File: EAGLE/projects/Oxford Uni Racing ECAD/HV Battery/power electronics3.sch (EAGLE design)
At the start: 57 parts, among them IC1 4043N, IC2 4001N, IC3 LM555CN, IC4 4071N, IC5 4081N, IC6 4011N, IC7 4011N, K1 T9AS1D12-48=T9A, K2 T9AS5D12-12=T9A, K4 T9AS1D12-48=T9A, K5 T9AS1D12-48=T9A, Q1 BS170, Q2 BS170, Q3 BS170

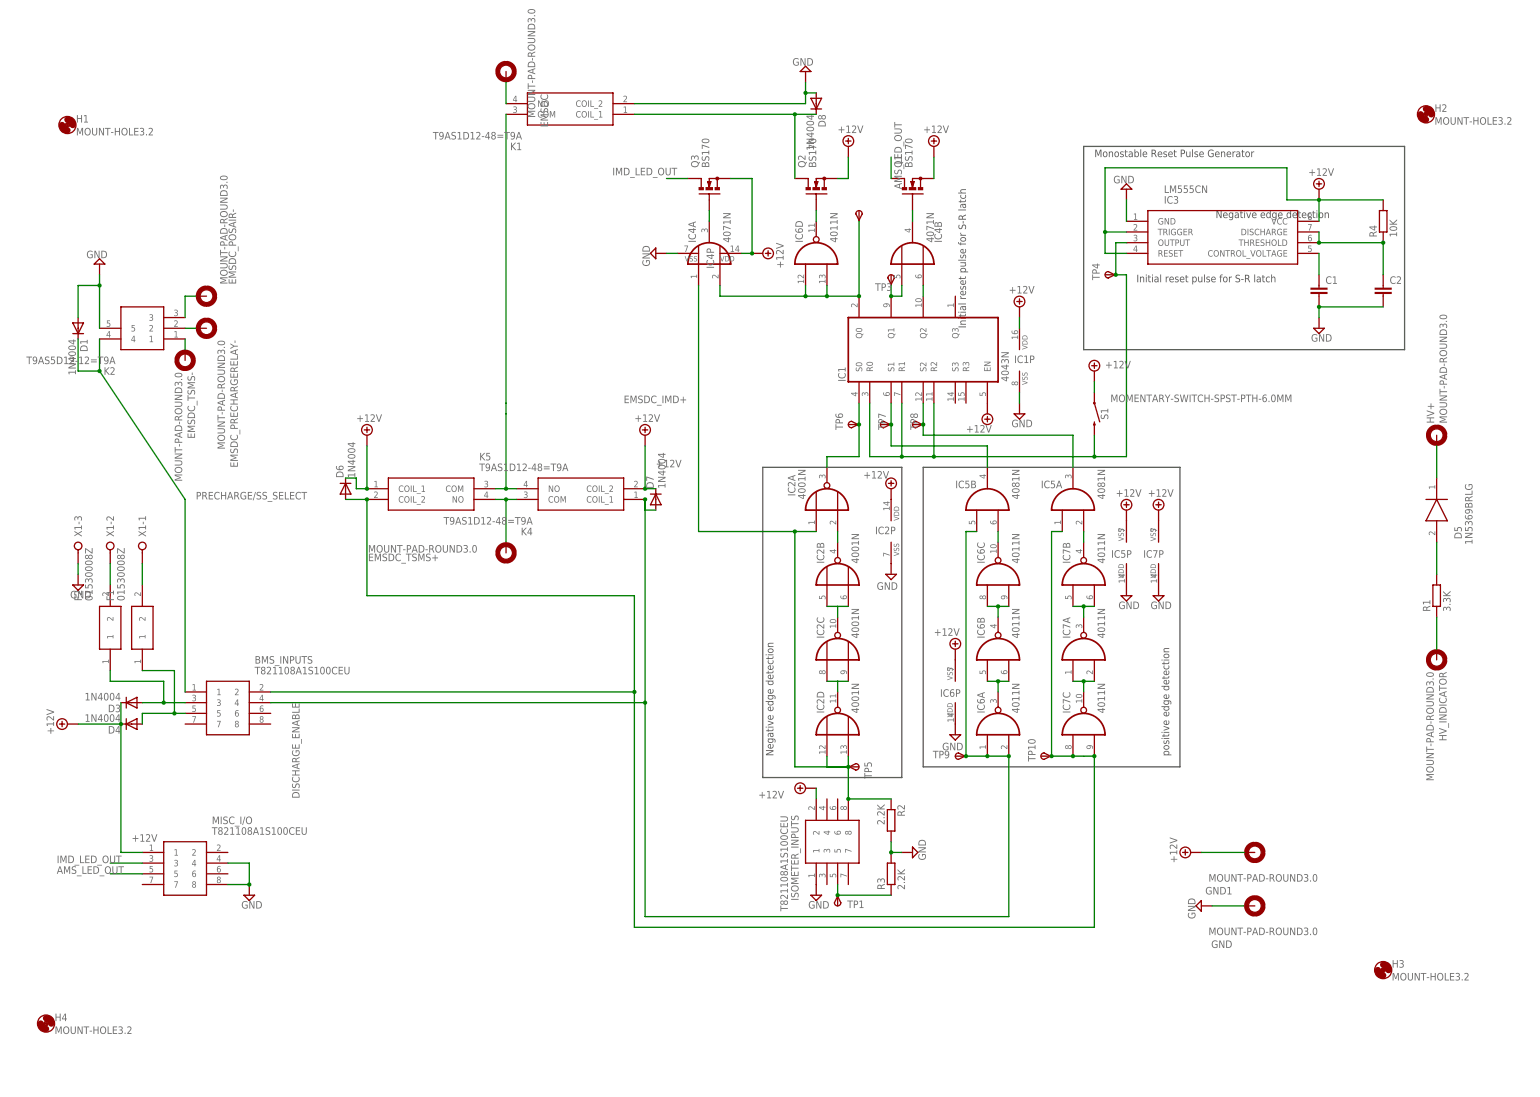
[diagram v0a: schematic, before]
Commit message: Modifications suggested by Dan after first review
Signed-off-by: Jack Bruford <jack.bruford41@gmail.com>
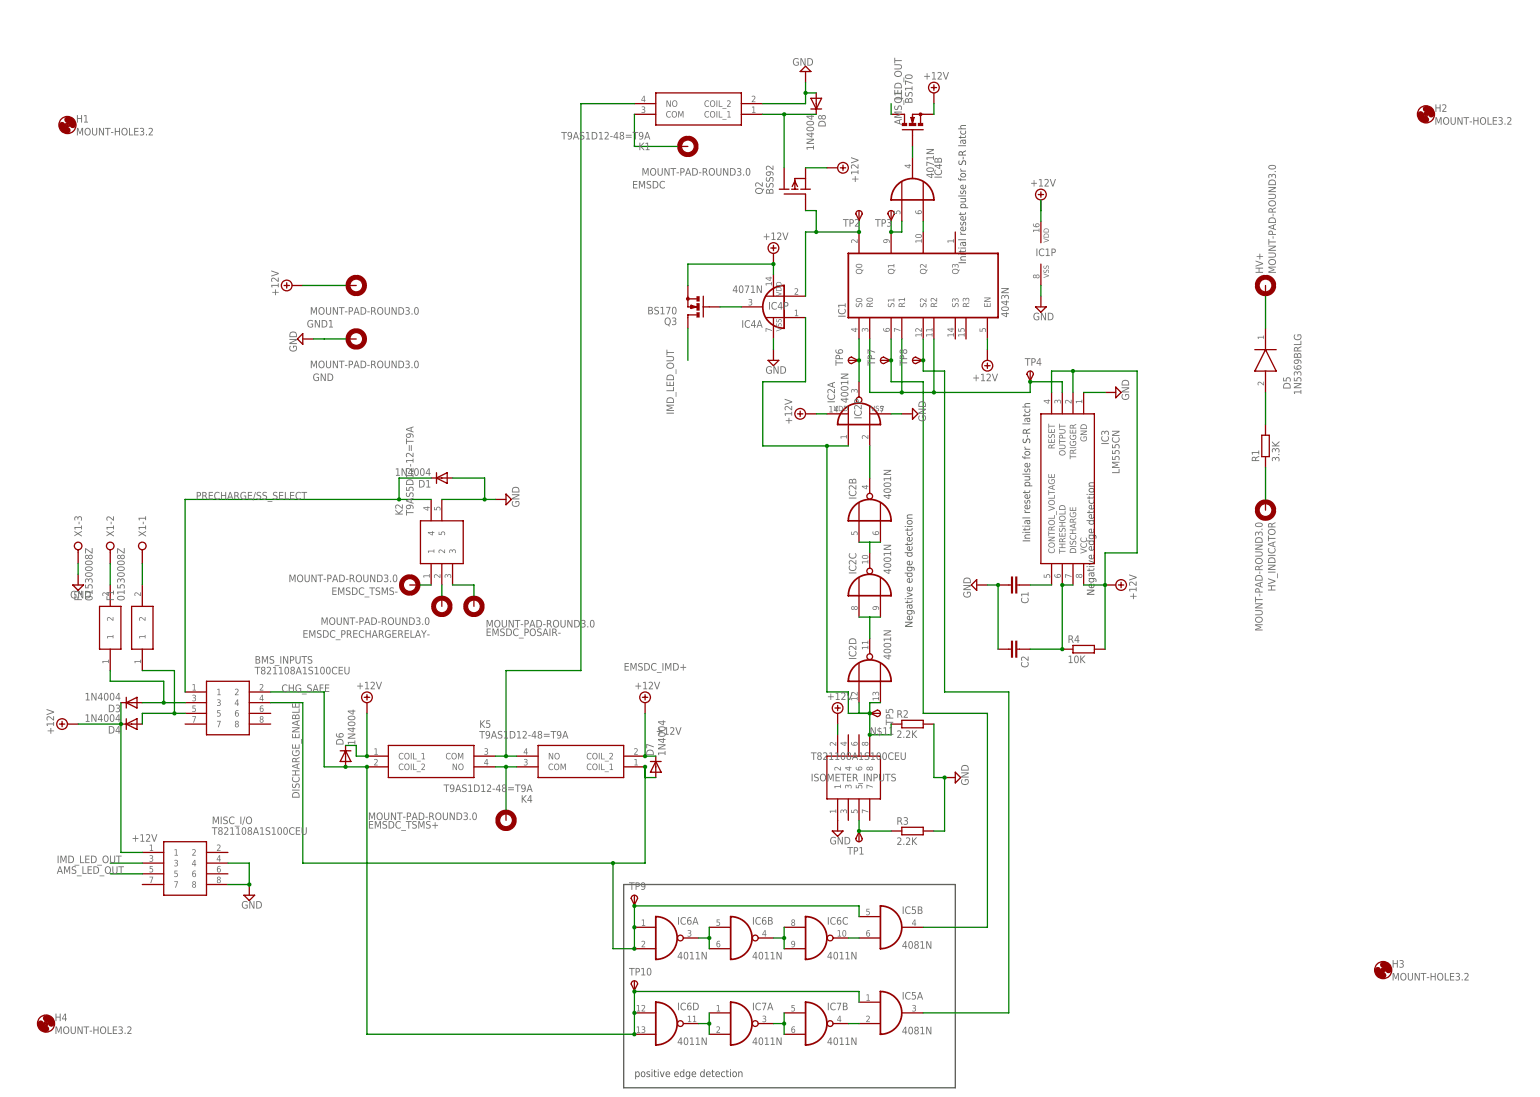
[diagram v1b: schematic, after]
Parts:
- removed S1: MOMENTARY-SWITCH-SPST-PTH-6.0MM, SparkFun-Switches:MOMENTARY-SWITCH-SPST-PTH-6.0MM
- Q2: value BS170 -> BSS92; device transistor-small-signal:BS170 -> transistor-fet:BSS92
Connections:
- removed net N$36: IC5A.I0, IC7C.I0, TP10.PP
- removed net N$37: IC6D.O, Q2.G
- net +12V: no longer IC5P.VSS, IC6P.VSS, IC7P.VSS, S1.1
- net CHG_SAFE: now also IC5A.I0, IC6D.I0, IC6D.I1, TP10.PP; no longer IC7C.I1
- net EMSDC_IMD+: now also K1.NO; no longer K1.COM
- net GND: no longer IC5P.VDD, IC6P.VDD, IC7P.VDD
- net N$16: now also K1.COM; no longer K1.NO
- net N$20: no longer S1.2
- net N$21: now also Q2.G; no longer IC6D.I0, IC6D.I1
- net N$32: now also IC6D.O; no longer IC7C.O
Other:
- note removed: "Monostable Reset Pulse Generator"
- moved on the sheet: C1, C2, D1, D5, D6, D7, EMSDC, EMSDC_POSAIR-, EMSDC_PRECHARGERELAY-, EMSDC_TSMS+, EMSDC_TSMS-, GND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
